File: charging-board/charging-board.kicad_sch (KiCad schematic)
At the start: 56 parts, among them J1 Conn_02x13_Counter_Clockwise, J10 TSMP_to_Banana Jacks, J12 everything_connector, J13 FTSH-107-01-F-DV-K-P-TR, J2 Conn_01x04, J8 J1772_Negotiation, J9 TSMP_to_HV, K1 RELAY_PR30-12V-450-1A-E, SW1 Y97KT23B5NAFP, U1 AP63205WU, U2 ISO1044BD, U3 STM32G441KBTx, U7 MIC5504-3.3YM5, Y2 ECS-240-8-37B-CKY-TR

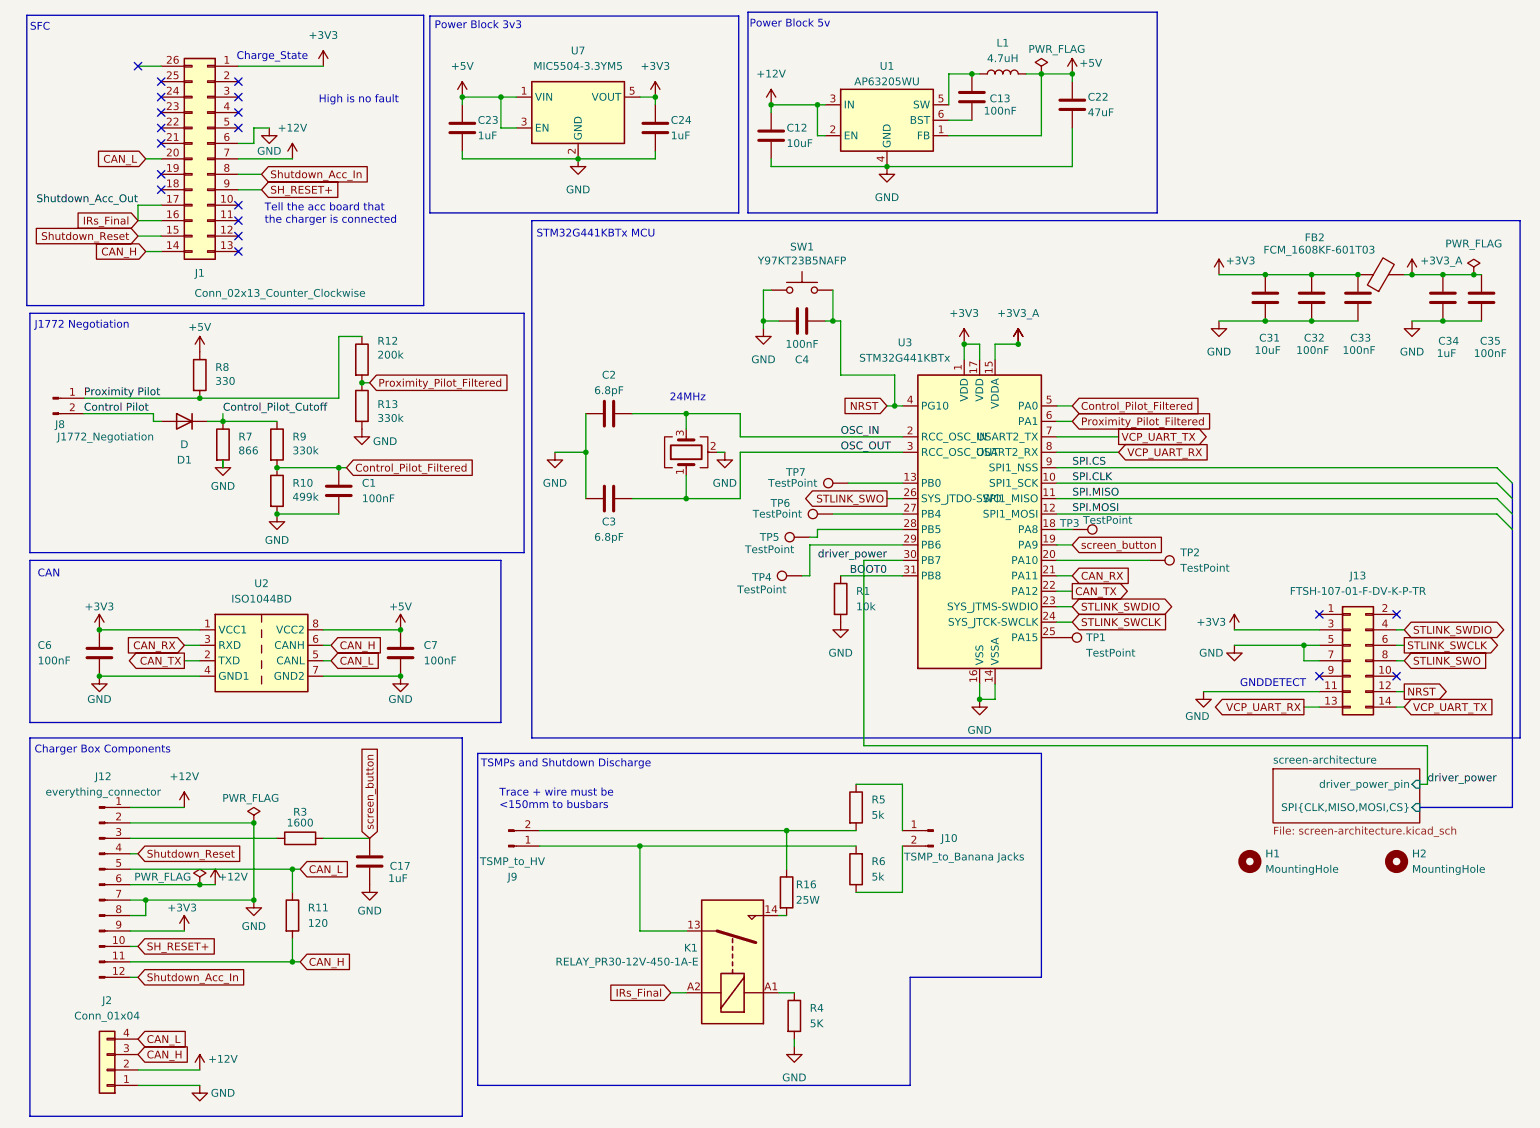
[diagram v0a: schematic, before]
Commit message: minor changes
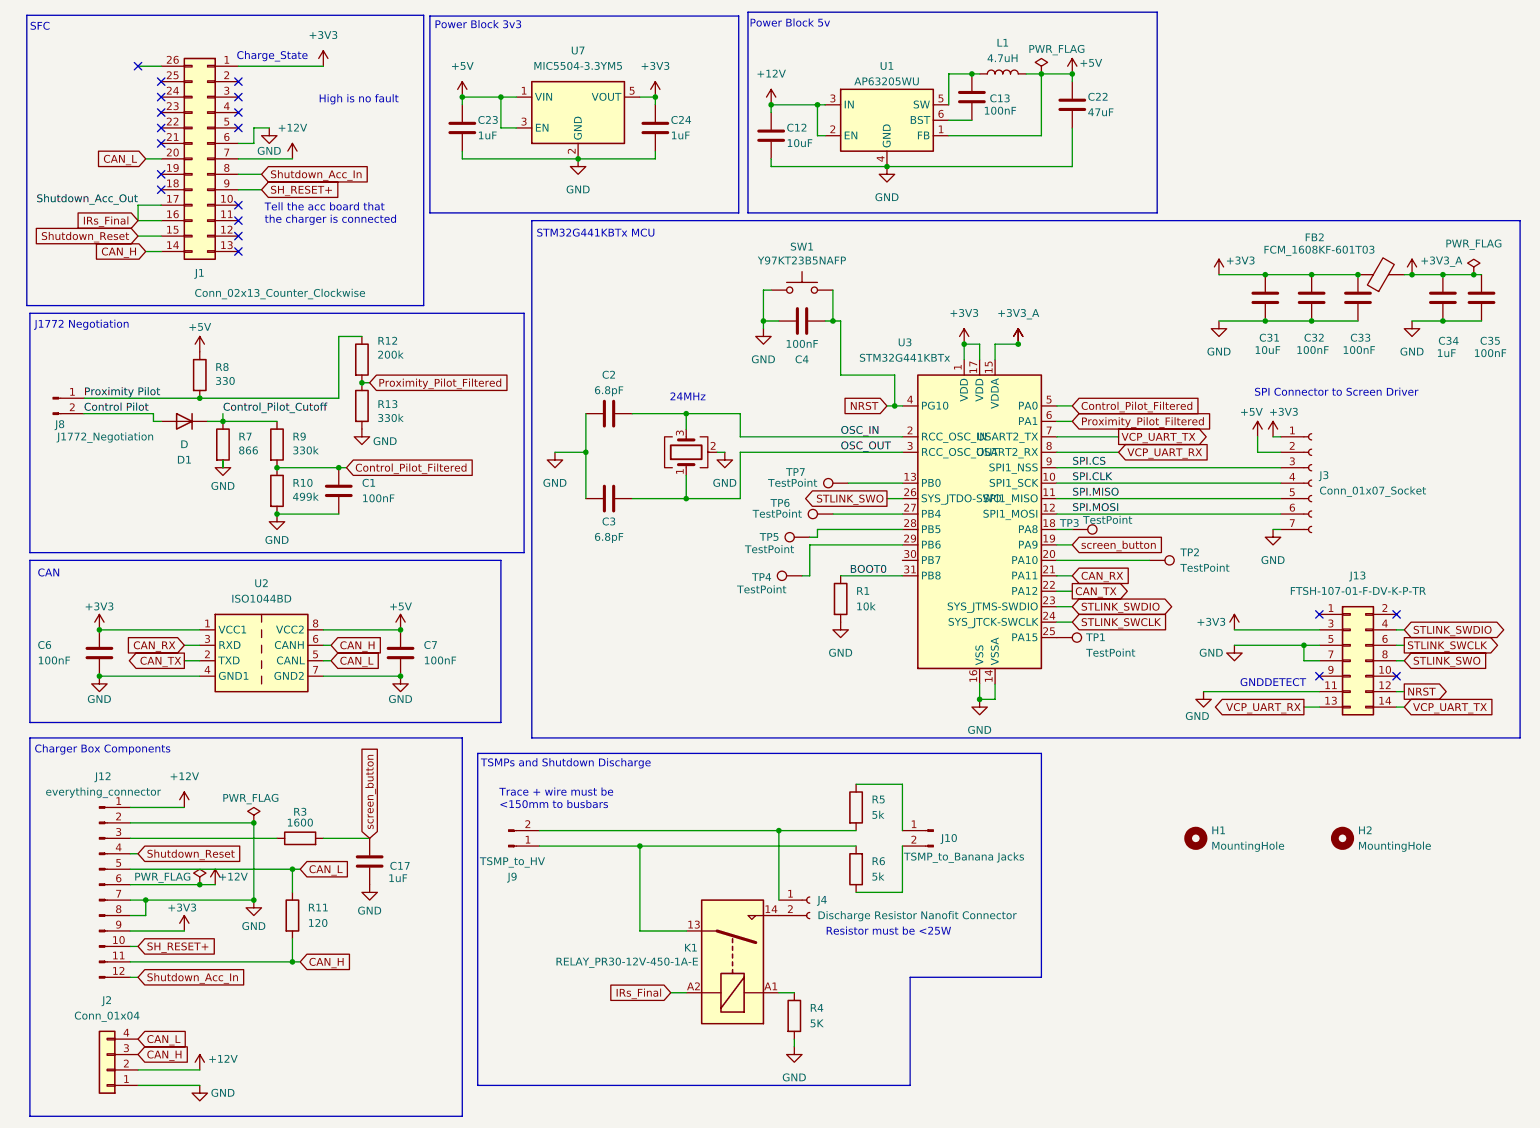
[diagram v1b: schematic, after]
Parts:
- removed R16: 25W, symbol Device:R
- added J3: Conn_01x07_Socket, Connector_FFC-FPC:Molex_200528-0070_1x07-1MP_P1.00mm_Horizontal, symbol Connector:Conn_01x07_Socket
- added J4: Discharge Resistor Nanofit Connector, Connector_Molex:Molex_Nano-Fit_105313-xx02_1x02_P2.50mm_Horizontal, symbol Connector:Conn_01x02_Socket
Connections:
- net +3V3: now also J3.1 (Pin_1)
- net +5V: now also J3.2 (Pin_2)
- net GND: now also J3.7 (Pin_7)
- net SPI.CLK: now also J3.4 (Pin_4)
- net SPI.CS: now also J3.3 (Pin_3)
- net SPI.MISO: now also J3.5 (Pin_5)
- net SPI.MOSI: now also J3.6 (Pin_6)
- net at J9.2 (Pin_2), R5.2: now also J4.1 (Pin_1)
- net at K1.14: now also J4.2 (Pin_2)
- net driver_power: no longer names the net of U3.30 (PB7)
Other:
- removed sheet screen-architecture
- note added: "Resistor must be <25W"
- note added: "SPI Connector to Screen Driver"
- moved on the sheet: H1, H2
